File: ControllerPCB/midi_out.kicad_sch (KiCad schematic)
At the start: 4 parts, among them J301 MIDI Out Conn, U301 74LVC1G17

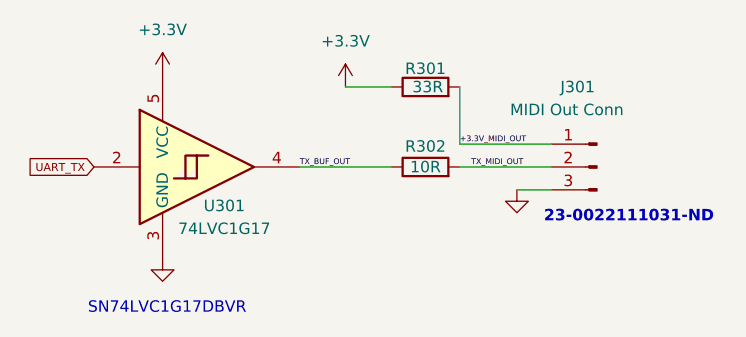
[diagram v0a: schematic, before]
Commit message: rev 0.3
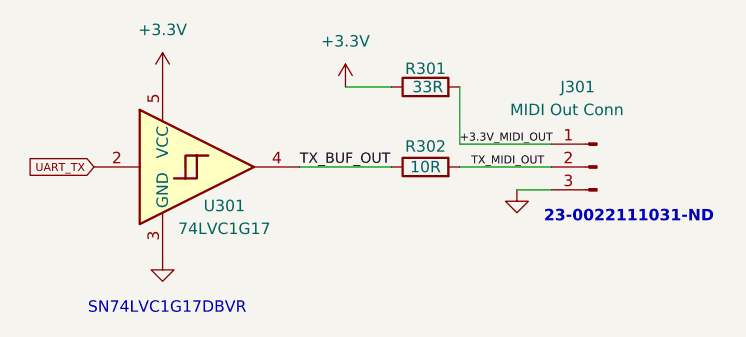
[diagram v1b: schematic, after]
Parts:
- J301: footprint 22292031:CONN_AE-6410-03A_MOL -> 0_Footprint_lib:CONN_AE-6410-03A_MOL
- U301: footprint SN74LVC1G17DBVR:SOT95P280X145-5N -> 0_Footprint_lib:SOT95P280X145-5N
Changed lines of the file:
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@@
 		(effects
 			(font
-				(size 0.635 0.635)
+				(size 0.889 0.889)
 			)
 			(justify left bottom)
@@
 		(effects
 			(font
-				(size 0.635 0.635)
+				(size 1.143 1.143)
 			)
 			(justify left bottom)
@@
 		(effects
 			(font
-				(size 0.635 0.635)
+				(size 0.889 0.889)
 			)
 			(justify left bottom)
@@
 			)
 		)
-		(property "Footprint" "22292031:CONN_AE-6410-03A_MOL"
+		(property "Footprint" "0_Footprint_lib:CONN_AE-6410-03A_MOL"
 			(at 121.92 59.69 0)
 			(effects
@@
 			)
 		)
-		(property "Footprint" "SN74LVC1G17DBVR:SOT95P280X145-5N"
+		(property "Footprint" "0_Footprint_lib:SOT95P280X145-5N"
 			(at 76.2 59.69 0)
 			(effects
